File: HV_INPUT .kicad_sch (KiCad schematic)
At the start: 11 parts, among them J1 928814-1, J6 928814-1, J7 928814-1

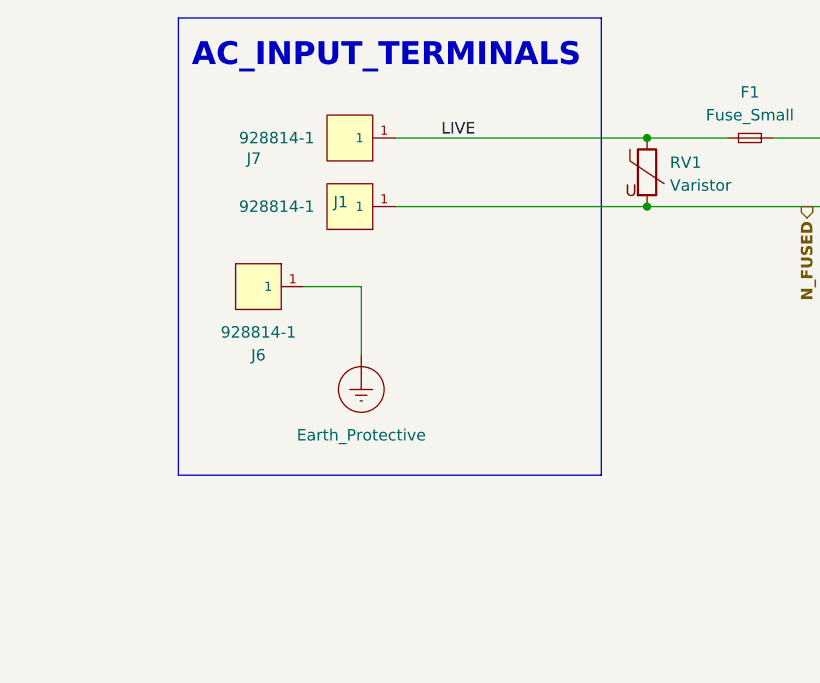
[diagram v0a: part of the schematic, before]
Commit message: Updated PCB files
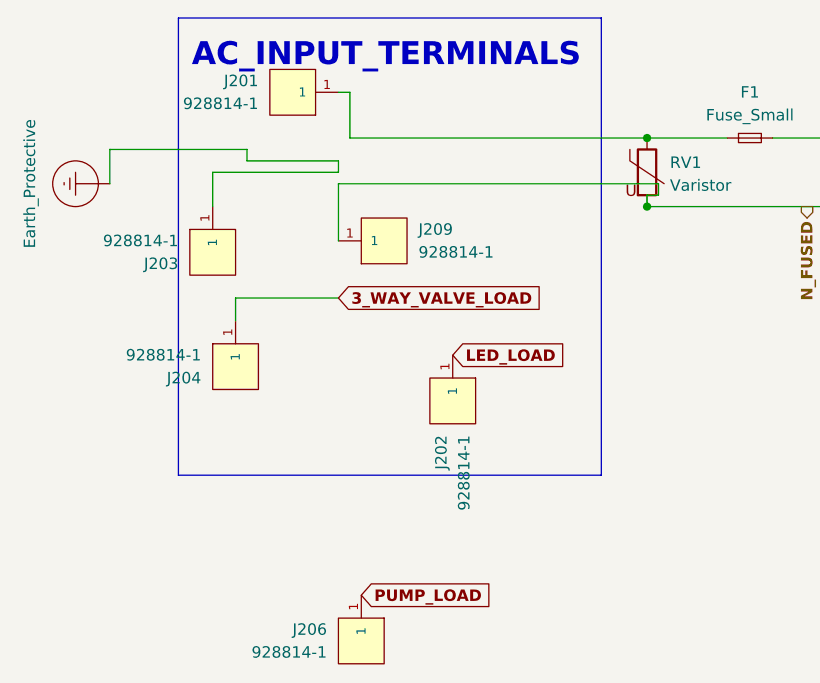
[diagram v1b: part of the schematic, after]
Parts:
- removed J1, J6, J7: 928814-1, 6.3mm spade:TE_928814-1, symbol 6.3mm spade:928814-1
- added J201, J202, J203, J204, J206, J209: 928814-1, 6.3mm spade:TE_928814-1, symbol 6.3mm spade:928814-1
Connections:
- net Earth_Protective: now also J203.1
- net N_FUSED: now also J209.1
- net LIVE: no longer names the net of F1.1, RV1.1
- net LIVE: now also J201.1
- new net 3_WAY_VALVE_LOAD: J204.1
- new net LED_LOAD: J202.1
- new net PUMP_LOAD: J206.1
